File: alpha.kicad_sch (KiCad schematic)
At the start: 22 parts, among them SW1 SW_Push, U1 ESP32-S3-PICO-1-N8R2, U2 AD620, Y1 Crystal

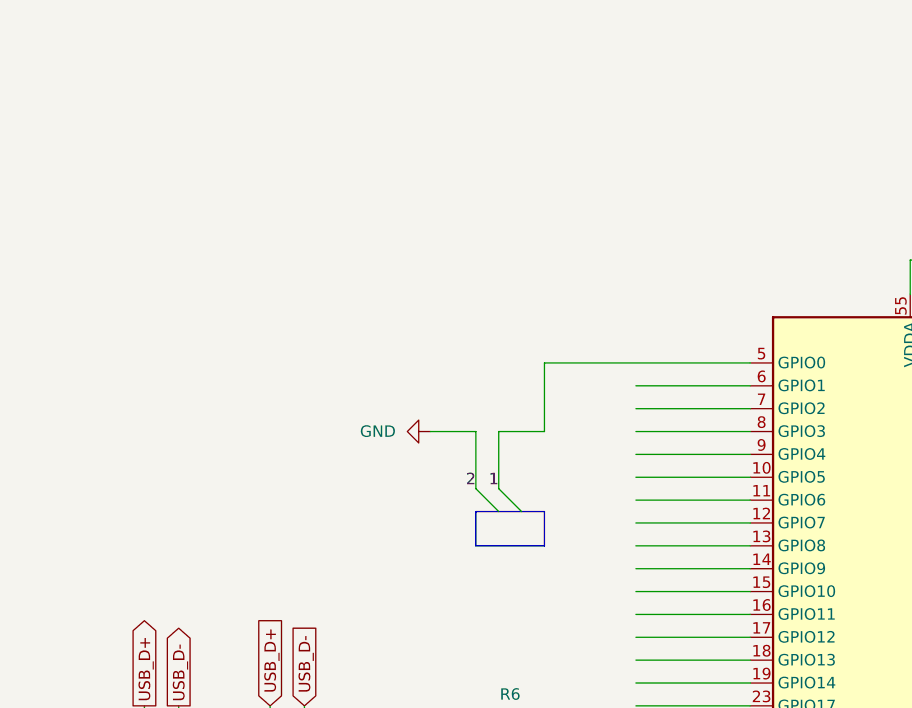
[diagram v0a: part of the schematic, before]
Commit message: Added Anaog Schematics
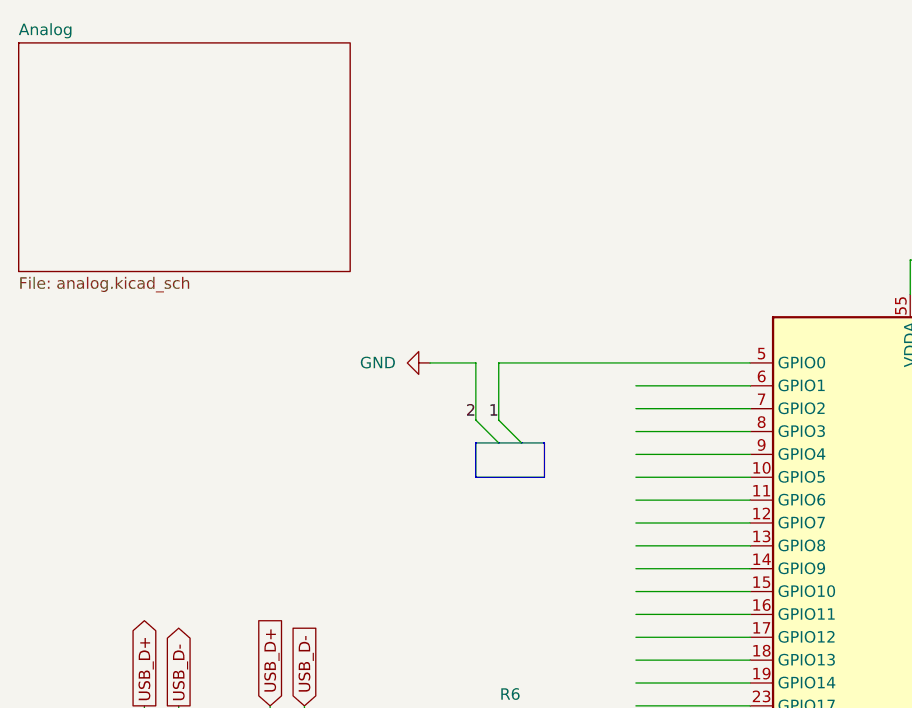
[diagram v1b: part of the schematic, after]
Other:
- added sheet Analog (analog.kicad_sch)
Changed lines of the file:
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@@
 	(generator "eeschema")
 	(generator_version "8.0")
-	(paper "A3")
+	(paper "A4")
 	(title_block
 		(title "Wireless ECG(ESDP 2024)")
@@
 	)
 	(bus_entry
-		(at 72.39 66.04)
+		(at 72.39 58.42)
 		(size 2.54 2.54)
 		(stroke
@@
 	)
 	(bus_entry
-		(at 69.85 66.04)
+		(at 69.85 58.42)
 		(size 2.54 2.54)
 		(stroke
@@
 	(wire
 		(pts
-			(xy 69.85 66.04) (xy 69.85 59.69)
+			(xy 69.85 58.42) (xy 69.85 52.07)
 		)
 		(stroke
@@
 	(wire
 		(pts
-			(xy 77.47 52.07) (xy 77.47 59.69)
-		)
-		(stroke
-			(width 0)
-			(type default)
-		)
-	)
-	(wire
-		(pts
 			(xy 87.63 64.77) (xy 100.33 64.77)
 		)
@@
 	(wire
 		(pts
-			(xy 72.39 59.69) (xy 72.39 66.04)
+			(xy 72.39 52.07) (xy 72.39 58.42)
 		)
 		(stroke
@@
 	(bus
 		(pts
-			(xy 69.85 68.58) (xy 72.39 68.58)
+			(xy 69.85 60.96) (xy 72.39 60.96)
 		)
 		(stroke
@@
 	(wire
 		(pts
-			(xy 77.47 59.69) (xy 72.39 59.69)
+			(xy 72.39 52.07) (xy 100.33 52.07)
 		)
 		(stroke
@@
 	(wire
 		(pts
-			(xy 100.33 52.07) (xy 77.47 52.07)
-		)
-		(stroke
-			(width 0)
-			(type default)
-		)
-	)
-	(wire
-		(pts
 			(xy 68.58 100.33) (xy 68.58 97.79)
 		)
@@
 	(bus
 		(pts
-			(xy 77.47 68.58) (xy 77.47 72.39)
+			(xy 77.47 60.96) (xy 77.47 64.77)
 		)
 		(stroke
@@
 	(wire
 		(pts
-			(xy 64.77 59.69) (xy 69.85 59.69)
+			(xy 64.77 52.07) (xy 69.85 52.07)
 		)
 		(stroke
@@
 	(bus
 		(pts
-			(xy 72.39 68.58) (xy 74.93 68.58)
+			(xy 72.39 60.96) (xy 74.93 60.96)
 		)
 		(stroke
@@
 	(bus
 		(pts
-			(xy 69.85 68.58) (xy 69.85 72.39)
+			(xy 69.85 60.96) (xy 69.85 64.77)
 		)
 		(stroke
@@
 	(bus
 		(pts
-			(xy 74.93 68.58) (xy 77.47 68.58)
+			(xy 74.93 60.96) (xy 77.47 60.96)
 		)
 		(stroke
@@
 	(bus
 		(pts
-			(xy 77.47 72.39) (xy 69.85 72.39)
+			(xy 77.47 64.77) (xy 69.85 64.77)
 		)
 		(stroke
@@
 	)
 	(label "1"
-		(at 72.39 66.04 180)
+		(at 72.39 58.42 180)
 		(fields_autoplaced yes)
 		(effects
@@
 	)
 	(label "2"
-		(at 69.85 66.04 180)
+		(at 69.85 58.42 180)
 		(fields_autoplaced yes)
 		(effects
@@
 	(symbol
 		(lib_id "power:GND")
-		(at 64.77 59.69 270)
+		(at 64.77 52.07 270)
 		(unit 1)
 		(exclude_from_sim no)
@@
 		(fields_autoplaced yes)
 		(property "Reference" "#PWR05"
-			(at 58.42 59.69 0)
+			(at 58.42 52.07 0)
 			(effects
 				(font
@@
 		)
 		(property "Value" "GND"
-			(at 60.96 59.6899 90)
+			(at 60.96 52.0699 90)
 			(effects
 				(font
@@
 		)
 		(property "Footprint" ""
-			(at 64.77 59.69 0)
+			(at 64.77 52.07 0)
 			(effects
 				(font
@@
 		)
 		(property "Datasheet" ""
-			(at 64.77 59.69 0)
+			(at 64.77 52.07 0)
 			(effects
 				(font
@@
 		)
 		(property "Description" "Power symbol creates a global label with name \"GND\" , ground"
-			(at 64.77 59.69 0)
+			(at 64.77 52.07 0)
 			(effects
 				(font
@@
 				)
 			)
+		)
+	)
+	(sheet
+		(at 19.05 16.51)
+		(size 36.83 25.4)
+		(fields_autoplaced yes)
+		(stroke
+			(width 0.1524)
+			(type solid)
+		)
+		(fill
+			(color 0 0 0 0.0000)
+		)
+		(property "Sheetname" "Analog"
+			(at 19.05 15.7984 0)
+			(effects
+				(font
+					(size 1.27 1.27)
+				)
+				(justify left bottom)
+			)
+		)
+		(property "Sheetfile" "analog.kicad_sch"
+			(at 19.05 42.4946 0)
+			(effects
+				(font
+					(size 1.27 1.27)
+				)
+				(justify left top)
+			)
+		)
+		(instances
+			(project "alpha"
+				(path "/78da8bdf-e40e-495b-ba6c-b18ee9000176"
+					(page "2")
+				)
+			)

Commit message: Revert "Added Anaog Schematics"
This reverts commit a5de0399bf14b3a200f5f1346ef0d461a1e3e6ca.
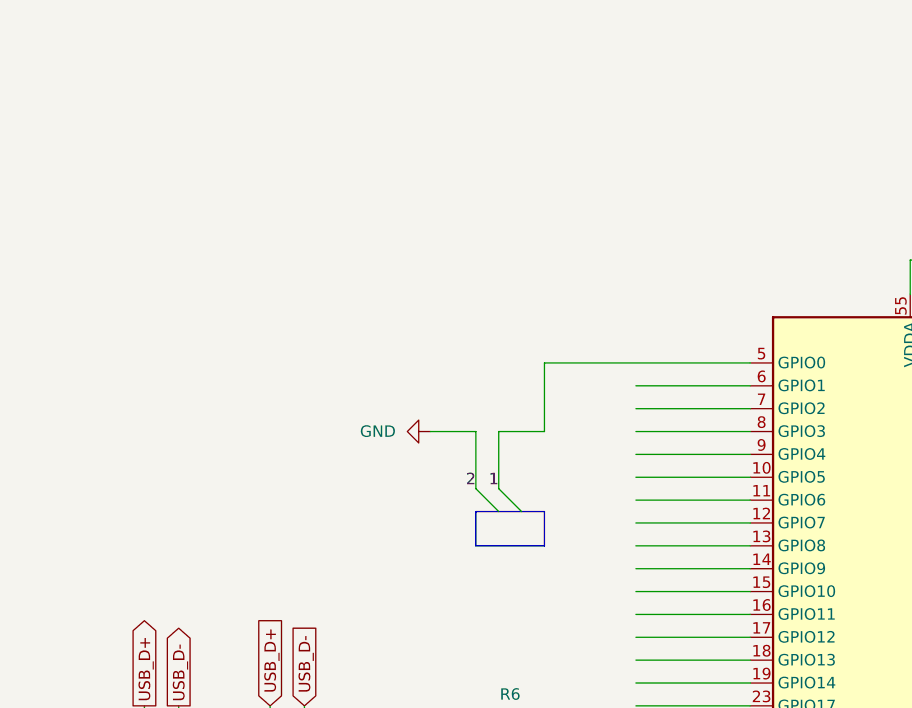
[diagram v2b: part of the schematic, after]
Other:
- removed sheet Analog
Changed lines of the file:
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@@
 	(generator "eeschema")
 	(generator_version "8.0")
-	(paper "A4")
+	(paper "A3")
 	(title_block
 		(title "Wireless ECG(ESDP 2024)")
@@
 	)
 	(bus_entry
-		(at 72.39 58.42)
+		(at 72.39 66.04)
 		(size 2.54 2.54)
 		(stroke
@@
 	)
 	(bus_entry
-		(at 69.85 58.42)
+		(at 69.85 66.04)
 		(size 2.54 2.54)
 		(stroke
@@
 	(wire
 		(pts
-			(xy 69.85 58.42) (xy 69.85 52.07)
+			(xy 69.85 66.04) (xy 69.85 59.69)
 		)
 		(stroke
@@
 	(wire
 		(pts
+			(xy 77.47 52.07) (xy 77.47 59.69)
+		)
+		(stroke
+			(width 0)
+			(type default)
+		)
+	)
+	(wire
+		(pts
 			(xy 87.63 64.77) (xy 100.33 64.77)
 		)
@@
 	(wire
 		(pts
-			(xy 72.39 52.07) (xy 72.39 58.42)
+			(xy 72.39 59.69) (xy 72.39 66.04)
 		)
 		(stroke
@@
 	(bus
 		(pts
-			(xy 69.85 60.96) (xy 72.39 60.96)
+			(xy 69.85 68.58) (xy 72.39 68.58)
 		)
 		(stroke
@@
 	(wire
 		(pts
-			(xy 72.39 52.07) (xy 100.33 52.07)
+			(xy 77.47 59.69) (xy 72.39 59.69)
 		)
 		(stroke
@@
 	(wire
 		(pts
+			(xy 100.33 52.07) (xy 77.47 52.07)
+		)
+		(stroke
+			(width 0)
+			(type default)
+		)
+	)
+	(wire
+		(pts
 			(xy 68.58 100.33) (xy 68.58 97.79)
 		)
@@
 	(bus
 		(pts
-			(xy 77.47 60.96) (xy 77.47 64.77)
+			(xy 77.47 68.58) (xy 77.47 72.39)
 		)
 		(stroke
@@
 	(wire
 		(pts
-			(xy 64.77 52.07) (xy 69.85 52.07)
+			(xy 64.77 59.69) (xy 69.85 59.69)
 		)
 		(stroke
@@
 	(bus
 		(pts
-			(xy 72.39 60.96) (xy 74.93 60.96)
+			(xy 72.39 68.58) (xy 74.93 68.58)
 		)
 		(stroke
@@
 	(bus
 		(pts
-			(xy 69.85 60.96) (xy 69.85 64.77)
+			(xy 69.85 68.58) (xy 69.85 72.39)
 		)
 		(stroke
@@
 	(bus
 		(pts
-			(xy 74.93 60.96) (xy 77.47 60.96)
+			(xy 74.93 68.58) (xy 77.47 68.58)
 		)
 		(stroke
@@
 	(bus
 		(pts
-			(xy 77.47 64.77) (xy 69.85 64.77)
+			(xy 77.47 72.39) (xy 69.85 72.39)
 		)
 		(stroke
@@
 	)
 	(label "1"
-		(at 72.39 58.42 180)
+		(at 72.39 66.04 180)
 		(fields_autoplaced yes)
 		(effects
@@
 	)
 	(label "2"
-		(at 69.85 58.42 180)
+		(at 69.85 66.04 180)
 		(fields_autoplaced yes)
 		(effects
@@
 	(symbol
 		(lib_id "power:GND")
-		(at 64.77 52.07 270)
+		(at 64.77 59.69 270)
 		(unit 1)
 		(exclude_from_sim no)
@@
 		(fields_autoplaced yes)
 		(property "Reference" "#PWR05"
-			(at 58.42 52.07 0)
+			(at 58.42 59.69 0)
 			(effects
 				(font
@@
 		)
 		(property "Value" "GND"
-			(at 60.96 52.0699 90)
+			(at 60.96 59.6899 90)
 			(effects
 				(font
@@
 		)
 		(property "Footprint" ""
-			(at 64.77 52.07 0)
+			(at 64.77 59.69 0)
 			(effects
 				(font
@@
 		)
 		(property "Datasheet" ""
-			(at 64.77 52.07 0)
+			(at 64.77 59.69 0)
 			(effects
 				(font
@@
 		)
 		(property "Description" "Power symbol creates a global label with name \"GND\" , ground"
-			(at 64.77 52.07 0)
+			(at 64.77 59.69 0)
 			(effects
 				(font
@@
 				)
 			)
-		)
-	)
-	(sheet
-		(at 19.05 16.51)
-		(size 36.83 25.4)
-		(fields_autoplaced yes)
-		(stroke
-			(width 0.1524)
-			(type solid)
-		)
-		(fill
-			(color 0 0 0 0.0000)
-		)
-		(property "Sheetname" "Analog"
-			(at 19.05 15.7984 0)
-			(effects
-				(font
-					(size 1.27 1.27)
-				)
-				(justify left bottom)
-			)
-		)
-		(property "Sheetfile" "analog.kicad_sch"
-			(at 19.05 42.4946 0)
-			(effects
-				(font
-					(size 1.27 1.27)
-				)
-				(justify left top)
-			)
-		)
-		(instances
-			(project "alpha"
-				(path "/78da8bdf-e40e-495b-ba6c-b18ee9000176"
-					(page "2")
-				)
-			)
